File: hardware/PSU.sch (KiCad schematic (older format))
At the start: 6 parts

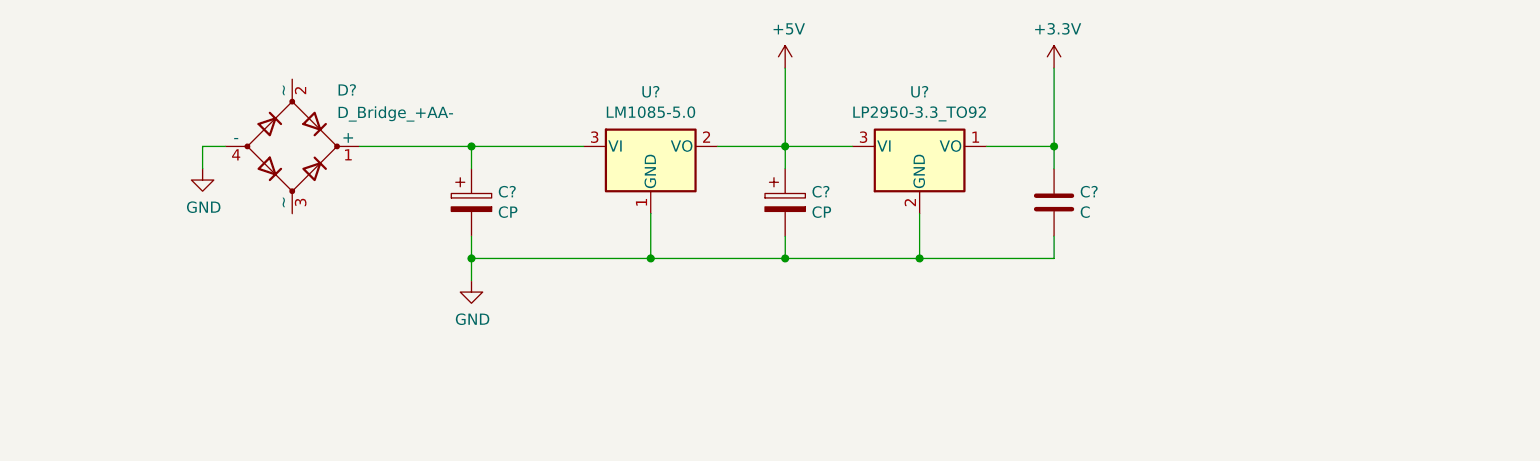
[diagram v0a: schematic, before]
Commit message: Updated PCB
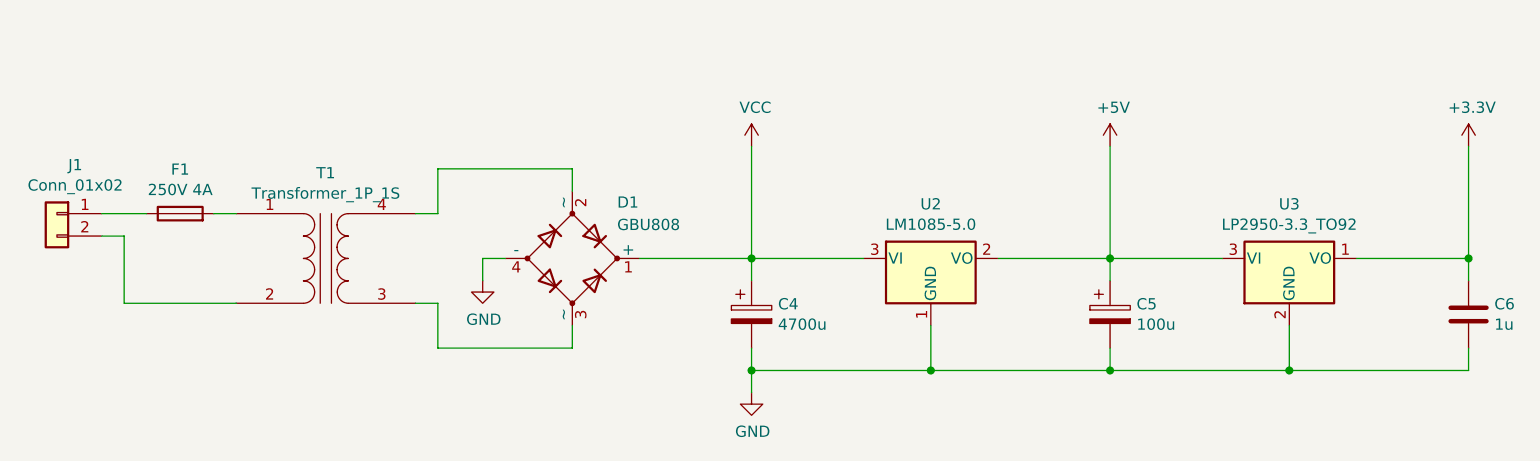
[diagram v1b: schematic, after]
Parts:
- added F1: 250V 4A, Fuse:Fuseholder_Cylinder-5x20mm_Schurter_0031_8201_Horizontal_Open, symbol Device:Fuse
- added J1: Conn_01x02, symbol Connector_Generic:Conn_01x02
- added T1: Transformer_1P_1S, symbol Device:Transformer_1P_1S
- C4: renamed from C?; value CP -> 4700u; footprint (none) -> Capacitor_THT:CP_Radial_D16.0mm_P7.50mm
- C5: renamed from C?; value CP -> 100u; footprint (none) -> Capacitor_THT:CP_Radial_D8.0mm_P3.50mm
- C6: renamed from C?; value C -> 1u; footprint (none) -> Capacitor_THT:C_Rect_L7.2mm_W4.5mm_P5.00mm_FKS2_FKP2_MKS2_MKP2
- D1: renamed from D?; value D_Bridge_+AA- -> GBU808; footprint Diode_THT:Diode_Bridge_Vishay_GBL -> Diode_THT:Diode_Bridge_Vishay_GBU
- gave numbers to parts that had none: 2
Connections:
- net VCC: now reaches C4.1, D1.1 (+), U2.3 (VI)
- net at D1.2 (~~): now also T1.4 (SB)
- net at D1.3 (~~): now also T1.3 (SA)
- new net: F1.2, T1.1 (AA)
- new net: J1.2 (Pin_2), T1.2 (AB)
- new net: F1.1, J1.1 (Pin_1)
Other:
- moved on the sheet: C4, C5, C6, D1, U2, U3
